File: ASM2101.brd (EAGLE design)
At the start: 16.5 x 16.5 mm, 19 parts, among them J1 GRPB032VWQS, J2 GRPB051VWCN, U1 ATMEGA328P-MU

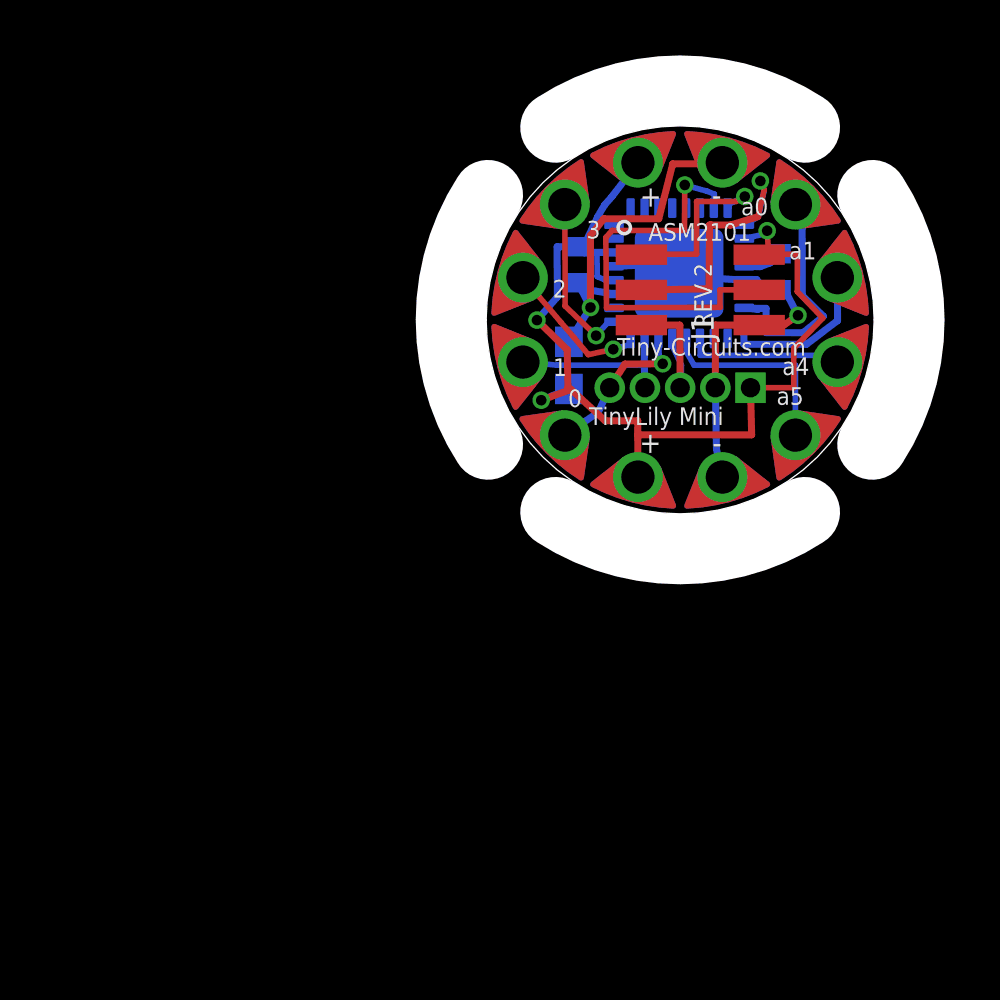
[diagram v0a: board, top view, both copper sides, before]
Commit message: Updated to Rev 3
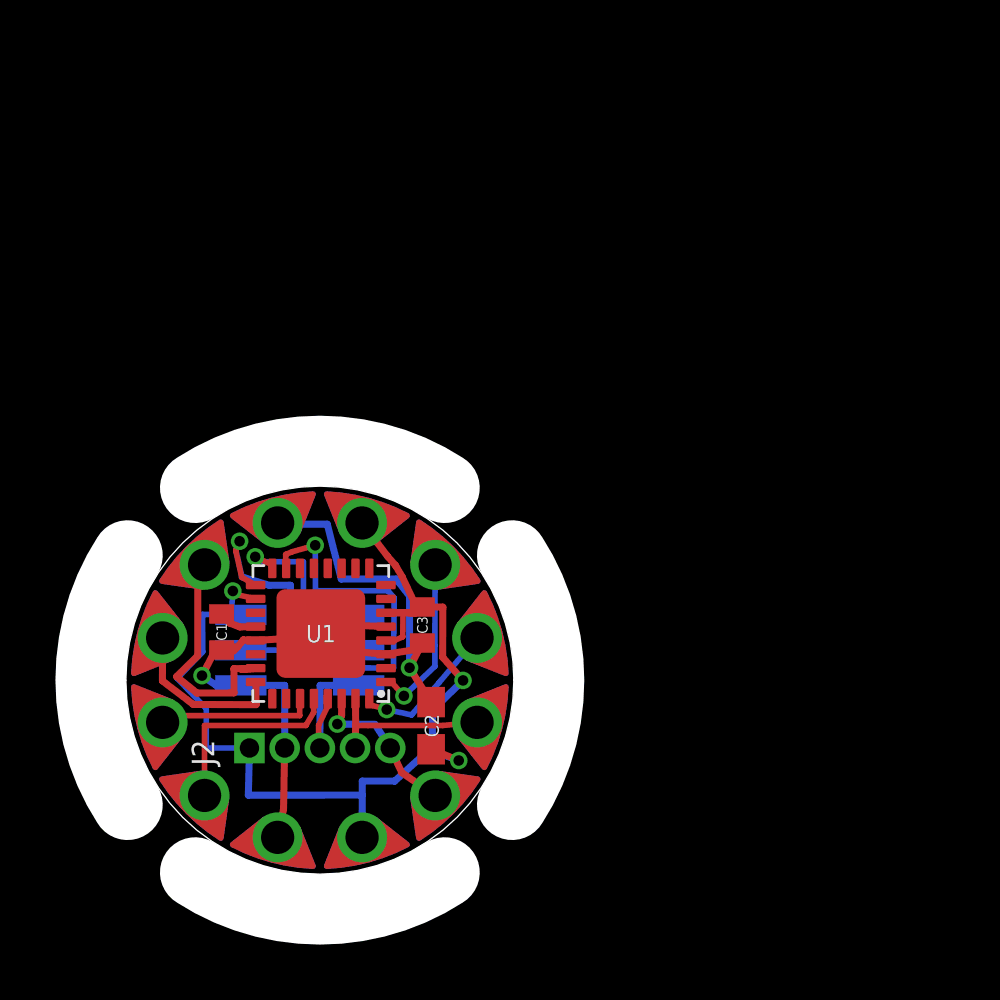
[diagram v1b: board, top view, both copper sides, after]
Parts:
- moved U$2 27.4 mm to (1.45, 5.51), flipped to the bottom
- moved U$3 27.4 mm to (1.45, 8.49), flipped to the bottom
- moved U$1 24.8 mm to (2.93, 2.93), flipped to the bottom
- moved U$4 24.8 mm to (2.93, 11.1), flipped to the bottom
- moved C1 23.9 mm to (3.45, 8.74), flipped to the top
- moved U$11 20.6 mm to (5.51, 1.45), flipped to the bottom
- moved U$12 20.6 mm to (5.51, 12.6), flipped to the bottom
- moved J1 19.4 mm to (6.27, 8.08), flipped to the bottom
- moved J2 18.4 mm to (7.00, 5.19), flipped to the top
- moved U1 18.3 mm to (7.03, 8.68), flipped to the top
- moved U$7 16.4 mm to (8.49, 1.45), flipped to the bottom
- moved U$8 16.4 mm to (8.49, 12.6), flipped to the bottom
- moved C3 14.2 mm to (10.7, 8.99), flipped to the top
- moved C2 13.9 mm to (11.0, 5.36), flipped to the top
- moved U$10 13.9 mm to (11.1, 2.93), flipped to the bottom
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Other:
- board text added: "REV 3"
- board text removed: "REV 2"
